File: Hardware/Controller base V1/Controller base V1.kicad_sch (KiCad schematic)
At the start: 30 parts, among them J1 USB_C_Receptacle_USB2.0_16P, J2 Conn_01x05_Pin, J7 Conn_02x10_Counter_Clockwise, J8 Conn_02x10_Counter_Clockwise, SW4 SW_Push, U1 AZ1117CH-3.3TRG1, U2 ESP32-S3-WROOM-1U-N4

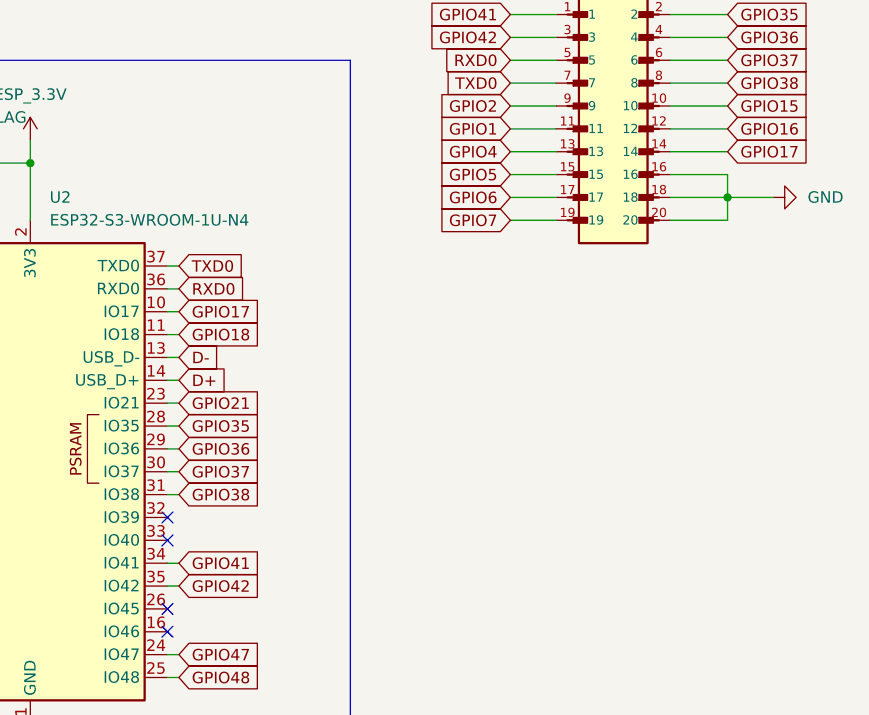
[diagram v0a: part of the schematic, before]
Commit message: update
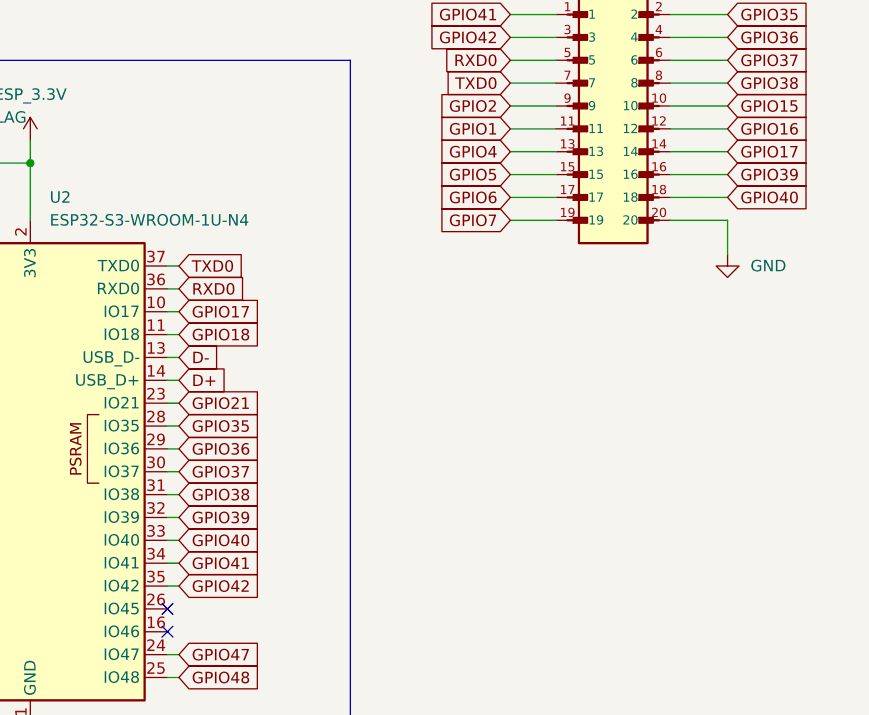
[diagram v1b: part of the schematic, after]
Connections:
- net GND: no longer J8.16, J8.18
- net GPIO39: now reaches U2.32 (IO39)
- net GPIO39: now also J8.16
- net GPIO40: now reaches U2.33 (IO40)
- net GPIO40: now also J8.18
- no-connect marks 6 -> 4
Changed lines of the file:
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@@
 	)
 	(junction
-		(at 271.78 91.44)
-		(diameter 0)
-		(color 0 0 0 0)
-	)
-	(junction
 		(at 157.48 31.75)
 		(diameter 0)
@@
 	)
 	(no_connect
-		(at 209.55 127)
-	)
-	(no_connect
 		(at 48.26 64.77)
 	)
 	(no_connect
-		(at 209.55 129.54)
-	)
-	(no_connect
 		(at 48.26 62.23)
 	)
@@
 	(wire
 		(pts
-			(xy 21.59 163.83) (xy 29.21 163.83)
+			(xy 271.78 97.79) (xy 271.78 93.98)
 		)
 		(stroke
@@
 	(wire
 		(pts
-			(xy 102.87 31.75) (xy 115.57 31.75)
+			(xy 209.55 127) (xy 210.82 127)
 		)
 		(stroke
@@
 	(wire
 		(pts
-			(xy 210.82 132.08) (xy 209.55 132.08)
+			(xy 21.59 163.83) (xy 29.21 163.83)
 		)
 		(stroke
@@
 	(wire
 		(pts
-			(xy 154.94 152.4) (xy 154.94 144.78)
+			(xy 102.87 31.75) (xy 115.57 31.75)
 		)
 		(stroke
@@
 	(wire
 		(pts
-			(xy 176.53 134.62) (xy 179.07 134.62)
+			(xy 210.82 132.08) (xy 209.55 132.08)
 		)
 		(stroke
@@
 	(wire
 		(pts
-			(xy 81.28 189.23) (xy 87.63 189.23)
+			(xy 154.94 152.4) (xy 154.94 144.78)
 		)
 		(stroke
@@
 	(wire
 		(pts
-			(xy 271.78 88.9) (xy 271.78 91.44)
+			(xy 176.53 134.62) (xy 179.07 134.62)
+		)
+		(stroke
+			(width 0)
+			(type default)
+		)
+	)
+	(wire
+		(pts
+			(xy 81.28 189.23) (xy 87.63 189.23)
 		)
 		(stroke
@@
 	(wire
 		(pts
-			(xy 271.78 91.44) (xy 276.86 91.44)
-		)
-		(stroke
-			(width 0)
-			(type default)
-		)
-	)
-	(wire
-		(pts
 			(xy 247.65 83.82) (xy 252.73 83.82)
 		)
@@
 	(wire
 		(pts
+			(xy 209.55 129.54) (xy 210.82 129.54)
+		)
+		(stroke
+			(width 0)
+			(type default)
+		)
+	)
+	(wire
+		(pts
 			(xy 153.67 87.63) (xy 153.67 88.9)
 		)
@@
 	(wire
 		(pts
-			(xy 271.78 93.98) (xy 271.78 91.44)
-		)
-		(stroke
-			(width 0)
-			(type default)
-		)
-	)
-	(wire
-		(pts
 			(xy 170.18 31.75) (xy 170.18 34.29)
 		)
@@
 	(wire
 		(pts
-			(xy 265.43 88.9) (xy 271.78 88.9)
+			(xy 247.65 76.2) (xy 252.73 76.2)
 		)
 		(stroke
@@
 	(wire
 		(pts
-			(xy 247.65 76.2) (xy 252.73 76.2)
+			(xy 210.82 144.78) (xy 209.55 144.78)
 		)
 		(stroke
@@
 	(wire
 		(pts
-			(xy 210.82 144.78) (xy 209.55 144.78)
+			(xy 67.31 49.53) (xy 67.31 57.15)
 		)
 		(stroke
@@
 	(wire
 		(pts
-			(xy 67.31 49.53) (xy 67.31 57.15)
+			(xy 55.88 85.09) (xy 49.53 85.09)
 		)
 		(stroke
@@
 	(wire
 		(pts
-			(xy 55.88 85.09) (xy 49.53 85.09)
+			(xy 271.78 59.69) (xy 271.78 57.15)
 		)
 		(stroke
@@
 	(wire
 		(pts
-			(xy 271.78 59.69) (xy 271.78 57.15)
+			(xy 74.93 52.07) (xy 72.39 52.07)
 		)
 		(stroke
@@
 	(wire
 		(pts
-			(xy 74.93 52.07) (xy 72.39 52.07)
+			(xy 67.31 46.99) (xy 48.26 46.99)
 		)
 		(stroke
@@
 	(wire
 		(pts
-			(xy 67.31 46.99) (xy 48.26 46.99)
+			(xy 265.43 91.44) (xy 271.78 91.44)
 		)
 		(stroke
@@
 	(wire
 		(pts
-			(xy 59.69 34.29) (xy 59.69 57.15)
+			(xy 265.43 88.9) (xy 271.78 88.9)
 		)
 		(stroke
@@
 	(wire
 		(pts
-			(xy 271.78 54.61) (xy 271.78 52.07)
+			(xy 59.69 34.29) (xy 59.69 57.15)
 		)
 		(stroke
@@
 	(wire
 		(pts
-			(xy 53.34 80.01) (xy 49.53 80.01)
+			(xy 271.78 54.61) (xy 271.78 52.07)
 		)
 		(stroke
@@
 	(wire
 		(pts
-			(xy 49.53 179.07) (xy 58.42 179.07)
+			(xy 53.34 80.01) (xy 49.53 80.01)
 		)
 		(stroke
@@
 	(wire
 		(pts
-			(xy 81.28 186.69) (xy 87.63 186.69)
+			(xy 49.53 179.07) (xy 58.42 179.07)
 		)
 		(stroke
@@
 	(wire
 		(pts
-			(xy 132.08 41.91) (xy 132.08 46.99)
+			(xy 81.28 186.69) (xy 87.63 186.69)
 		)
 		(stroke
@@
 	(wire
 		(pts
-			(xy 265.43 91.44) (xy 271.78 91.44)
+			(xy 132.08 41.91) (xy 132.08 46.99)
 		)
 		(stroke
@@
 		)
 	)
+	(global_label "GPIO40"
+		(shape input)
+		(at 271.78 91.44 0)
+		(fields_autoplaced yes)
+		(effects
+			(font
+				(size 1.27 1.27)
+			)
+			(justify left)
+		)
+		(property "Intersheetrefs" "${INTERSHEET_REFS}"
+			(at 281.6595 91.44 0)
+			(effects
+				(font
+					(size 1.27 1.27)
+				)
+				(justify left)
+				(hide yes)
+			)
+		)
+	)
 	(global_label "GPIO11"
 		(shape input)
@@
 		)
 	)
+	(global_label "GPIO39"
+		(shape input)
+		(at 210.82 127 0)
+		(fields_autoplaced yes)
+		(effects
+			(font
+				(size 1.27 1.27)
+			)
+			(justify left)
+		)
+		(property "Intersheetrefs" "${INTERSHEET_REFS}"
+			(at 220.6995 127 0)
+			(effects
+				(font
+					(size 1.27 1.27)
+				)
+				(justify left)
+				(hide yes)
+			)
+		)
+	)
 	(global_label "GPIO4"
 		(shape input)
@@
 		)
 	)
+	(global_label "GPIO39"
+		(shape input)
+		(at 271.78 88.9 0)
+		(fields_autoplaced yes)
+		(effects
+			(font
+				(size 1.27 1.27)
+			)
+			(justify left)
+		)
+		(property "Intersheetrefs" "${INTERSHEET_REFS}"
+			(at 281.6595 88.9 0)
+			(effects
+				(font
+					(size 1.27 1.27)
+				)
+				(justify left)
+				(hide yes)
+			)
+		)
+	)
 	(global_label "GPIO8"
 		(shape input)
@@
 		)
 	)
+	(global_label "GPIO40"
+		(shape input)
+		(at 210.82 129.54 0)
+		(fields_autoplaced yes)
+		(effects
+			(font
+				(size 1.27 1.27)
+			)
+			(justify left)
+		)
+		(property "Intersheetrefs" "${INTERSHEET_REFS}"
+			(at 220.6995 129.54 0)
+			(effects
+				(font
+					(size 1.27 1.27)
+				)
+				(justify left)
+				(hide yes)
+			)
+		)
+	)
 	(global_label "GPIO38"
 		(shape input)
@@
 	(symbol
 		(lib_id "MCU_Controller:GND")
-		(at 276.86 91.44 90)
+		(at 271.78 97.79 0)
 		(unit 1)
 		(exclude_from_sim no)
@@
 		(fields_autoplaced yes)
 		(property "Reference" "#PWR030"
-			(at 283.21 91.44 0)
+			(at 271.78 104.14 0)
 			(effects
 				(font
@@
 		)
 		(property "Value" "GND"
-			(at 280.67 91.4399 90)
+			(at 274.32 99.0599 0)
 			(effects
 				(font
 					(size 1.27 1.27)
 				)
-				(justify right)
+				(justify left)
 			)
 		)
 		(property "Footprint" ""
-			(at 276.86 91.44 0)
+			(at 271.78 97.79 0)
 			(effects
 				(font
@@
 		)
 		(property "Datasheet" ""
-			(at 276.86 91.44 0)
+			(at 271.78 97.79 0)
 			(effects
 				(font
@@
 		)
 		(property "Description" "Power symbol creates a global label with name \"GND\" , ground"
-			(at 276.86 91.44 0)
+			(at 271.78 97.79 0)
 			(effects
 				(font
